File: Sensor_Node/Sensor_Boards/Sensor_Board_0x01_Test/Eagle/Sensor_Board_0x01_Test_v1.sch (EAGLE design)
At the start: 14 parts, among them J1 M04_SMD_90, J4 ARDUINO_ISP, U2 ATMEGA328P_TQFP, Y1 8MHZ

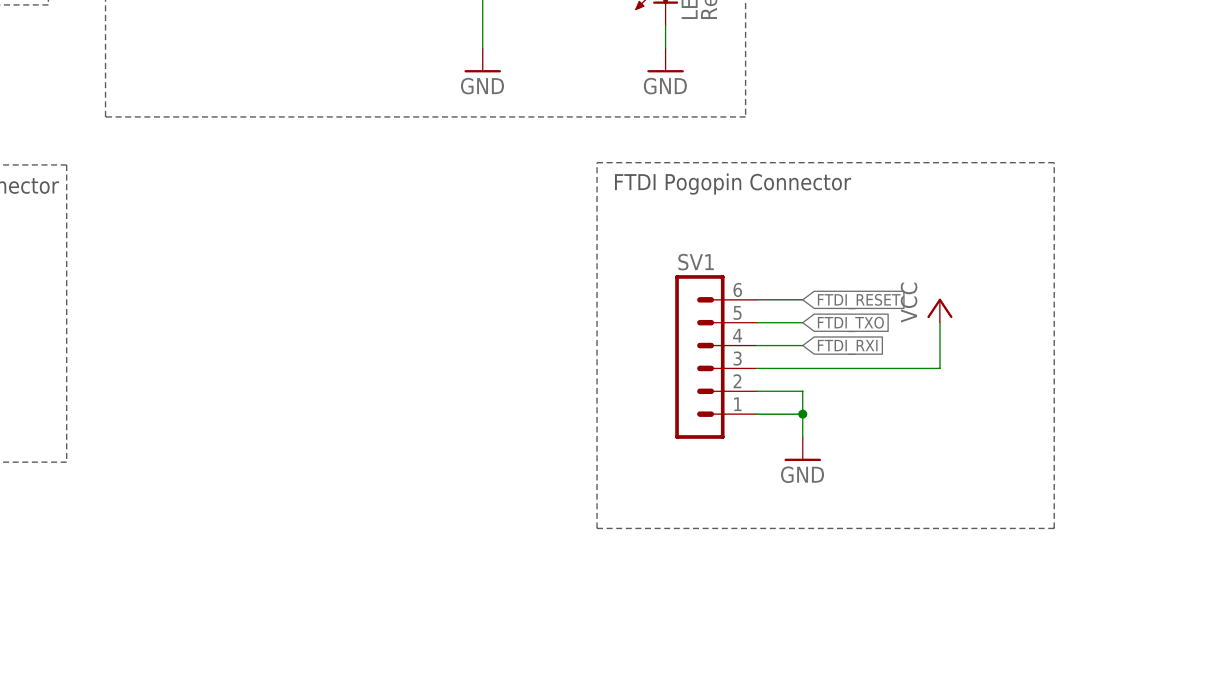
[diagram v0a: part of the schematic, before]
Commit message: Vorlage-Board fertig
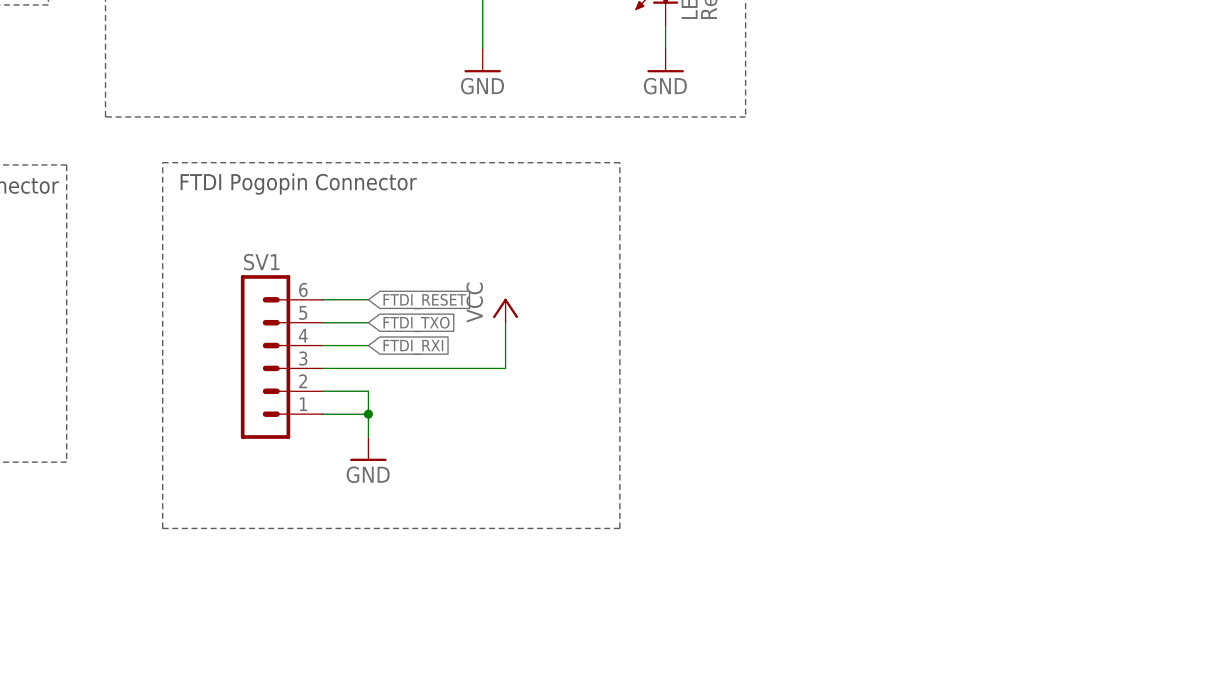
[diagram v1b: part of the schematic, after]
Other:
- moved on the sheet: SV1
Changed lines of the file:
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@@
 <text x="224.527240625" y="11.421534375" size="2.54" layer="94" font="vector">Sensor Board - SHT31 (0x02)</text>
 <text x="277.8550125" y="1.158059375" size="2.54" layer="94" font="vector">1.0</text>
-<wire x1="157.48" y1="63.5" x2="106.68" y2="63.5" width="0.1524" layer="97" style="shortdash"/>
-<wire x1="157.48" y1="22.86" x2="106.68" y2="22.86" width="0.1524" layer="97" style="shortdash"/>
-<wire x1="106.68" y1="22.86" x2="106.68" y2="63.5" width="0.1524" layer="97" style="shortdash"/>
-<wire x1="157.48" y1="22.86" x2="157.48" y2="63.5" width="0.1524" layer="97" style="shortdash"/>
-<text x="108.458" y="60.452" size="1.778" layer="97">FTDI Pogopin Connector</text>
+<wire x1="109.22" y1="63.5" x2="58.42" y2="63.5" width="0.1524" layer="97" style="shortdash"/>
+<wire x1="109.22" y1="22.86" x2="58.42" y2="22.86" width="0.1524" layer="97" style="shortdash"/>
+<wire x1="58.42" y1="22.86" x2="58.42" y2="63.5" width="0.1524" layer="97" style="shortdash"/>
+<wire x1="109.22" y1="22.86" x2="109.22" y2="63.5" width="0.1524" layer="97" style="shortdash"/>
+<text x="60.198" y="60.452" size="1.778" layer="97">FTDI Pogopin Connector</text>
 </plain>
 <instances>
@@
 <instance part="U$16" gate="G$1" x="106.68" y="88.9"/>
 <instance part="J1" gate="G$1" x="15.24" y="45.72" rot="MR180"/>
-<instance part="SV1" gate="1" x="116.84" y="43.18"/>
-<instance part="GND1" gate="1" x="129.54" y="30.48"/>
-<instance part="P+6" gate="VCC" x="144.78" y="48.26"/>
+<instance part="SV1" gate="1" x="68.58" y="43.18"/>
+<instance part="GND1" gate="1" x="81.28" y="30.48"/>
+<instance part="P+6" gate="VCC" x="96.52" y="48.26"/>
 <instance part="C1" gate="G$1" x="30.48" y="182.88" rot="R90"/>
 <instance part="U$1" gate="G$1" x="99.06" y="180.34"/>
@@
 <pinref part="SV1" gate="1" pin="1"/>
 <pinref part="GND1" gate="1" pin="GND"/>
-<wire x1="124.46" y1="35.56" x2="129.54" y2="35.56" width="0.1524" layer="91"/>
-<wire x1="129.54" y1="35.56" x2="129.54" y2="33.02" width="0.1524" layer="91"/>
+<wire x1="76.2" y1="35.56" x2="81.28" y2="35.56" width="0.1524" layer="91"/>
+<wire x1="81.28" y1="35.56" x2="81.28" y2="33.02" width="0.1524" layer="91"/>
 <pinref part="SV1" gate="1" pin="2"/>
-<wire x1="124.46" y1="38.1" x2="129.54" y2="38.1" width="0.1524" layer="91"/>
-<wire x1="129.54" y1="38.1" x2="129.54" y2="35.56" width="0.1524" layer="91"/>
-<junction x="129.54" y="35.56"/>
+<wire x1="76.2" y1="38.1" x2="81.28" y2="38.1" width="0.1524" layer="91"/>
+<wire x1="81.28" y1="38.1" x2="81.28" y2="35.56" width="0.1524" layer="91"/>
+<junction x="81.28" y="35.56"/>
 </segment>
 </net>
@@
 <pinref part="SV1" gate="1" pin="3"/>
 <pinref part="P+6" gate="VCC" pin="VCC"/>
-<wire x1="124.46" y1="40.64" x2="144.78" y2="40.64" width="0.1524" layer="91"/>
-<wire x1="144.78" y1="40.64" x2="144.78" y2="45.72" width="0.1524" layer="91"/>
+<wire x1="76.2" y1="40.64" x2="96.52" y2="40.64" width="0.1524" layer="91"/>
+<wire x1="96.52" y1="40.64" x2="96.52" y2="45.72" width="0.1524" layer="91"/>
 </segment>
 </net>
@@
 <segment>
 <pinref part="SV1" gate="1" pin="5"/>
-<wire x1="124.46" y1="45.72" x2="129.54" y2="45.72" width="0.1524" layer="91"/>
-<label x="129.54" y="45.72" size="1.27" layer="95" xref="yes"/>
+<wire x1="76.2" y1="45.72" x2="81.28" y2="45.72" width="0.1524" layer="91"/>
+<label x="81.28" y="45.72" size="1.27" layer="95" xref="yes"/>
 </segment>
 <segment>
@@
 <segment>
 <pinref part="SV1" gate="1" pin="4"/>
-<wire x1="124.46" y1="43.18" x2="129.54" y2="43.18" width="0.1524" layer="91"/>
-<label x="129.54" y="43.18" size="1.27" layer="95" xref="yes"/>
+<wire x1="76.2" y1="43.18" x2="81.28" y2="43.18" width="0.1524" layer="91"/>
+<label x="81.28" y="43.18" size="1.27" layer="95" xref="yes"/>
 </segment>
 <segment>
@@
 <segment>
 <pinref part="SV1" gate="1" pin="6"/>
-<wire x1="124.46" y1="48.26" x2="129.54" y2="48.26" width="0.1524" layer="91"/>
-<label x="129.54" y="48.26" size="1.27" layer="95" xref="yes"/>
-</segment>
-<segment>
+<wire x1="76.2" y1="48.26" x2="81.28" y2="48.26" width="0.1524" layer="91"/>
+<label x="81.28" y="48.26" size="1.27" layer="95" xref="yes"/>
+</segment>
+<segment>
